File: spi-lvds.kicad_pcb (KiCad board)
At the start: 2 copper layers, 39.9 x 34.9 mm, 8 parts

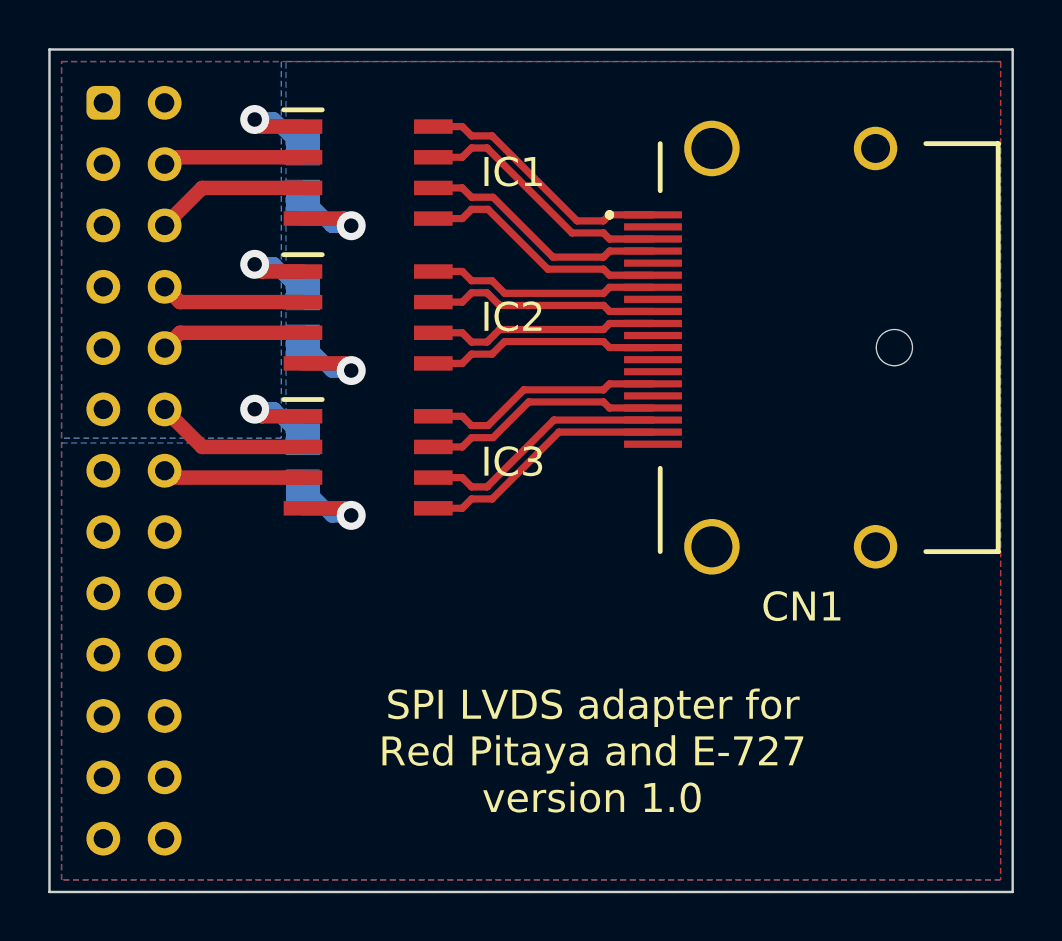
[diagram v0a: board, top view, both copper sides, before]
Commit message: improve GND and VCC
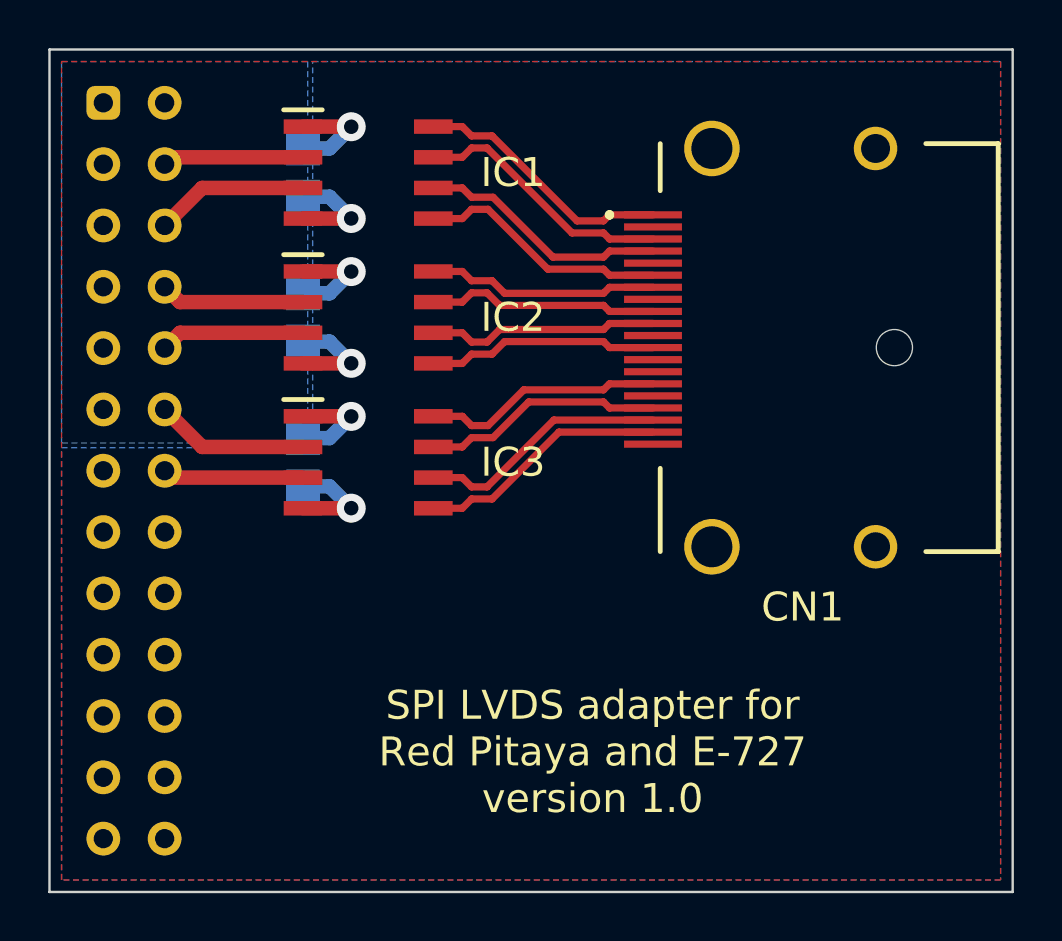
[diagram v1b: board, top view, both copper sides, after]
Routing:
- net VCC: track 13.9 -> 13.1 mm
- added copper zone on B.Cu, net GND
- removed copper zone on B.Cu, net (none)
